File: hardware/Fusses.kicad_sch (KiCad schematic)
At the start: 8 parts, among them U16 FOD8802DR2, U17 FOD8802DR2

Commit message: changed some footprints for clarity, and made some progress on board
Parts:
- removed D10, D9: D_SCH, Diode_SMD:D_0603_1608Metric, symbol Device:D_Schottky_Small
- removed R17, R18, R41, R42: R_Small, Resistor_SMD:R_0603_1608Metric, symbol Device:R_Small
- removed U16, U17: FOD8802DR2, SOIC127P600X175-8N, symbol FOD8802DR2:FOD8802DR2
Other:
- added sheet Supply (eFuse supply 24V.kicad_sch)
- note added: "Smart Fuses 24V"
- note added: "eFuses 24V"
- note added: "eFuses 5V"
- note removed: "Fuses"

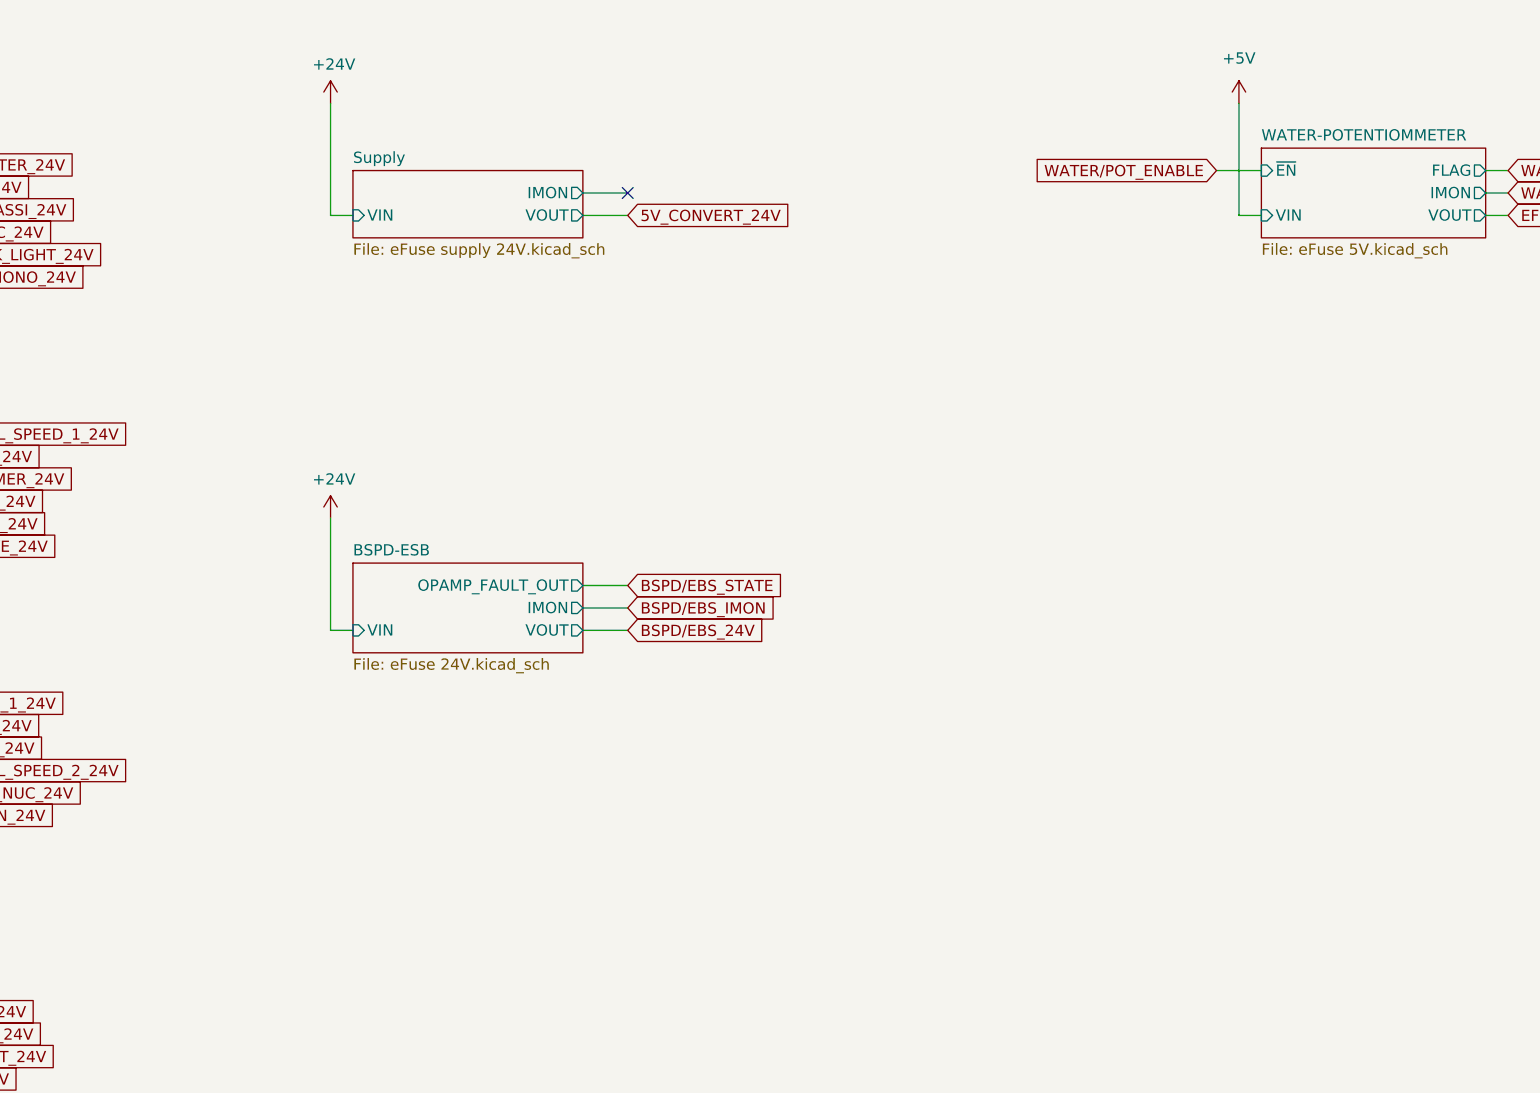
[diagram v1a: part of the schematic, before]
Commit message: finished new wersion of the board
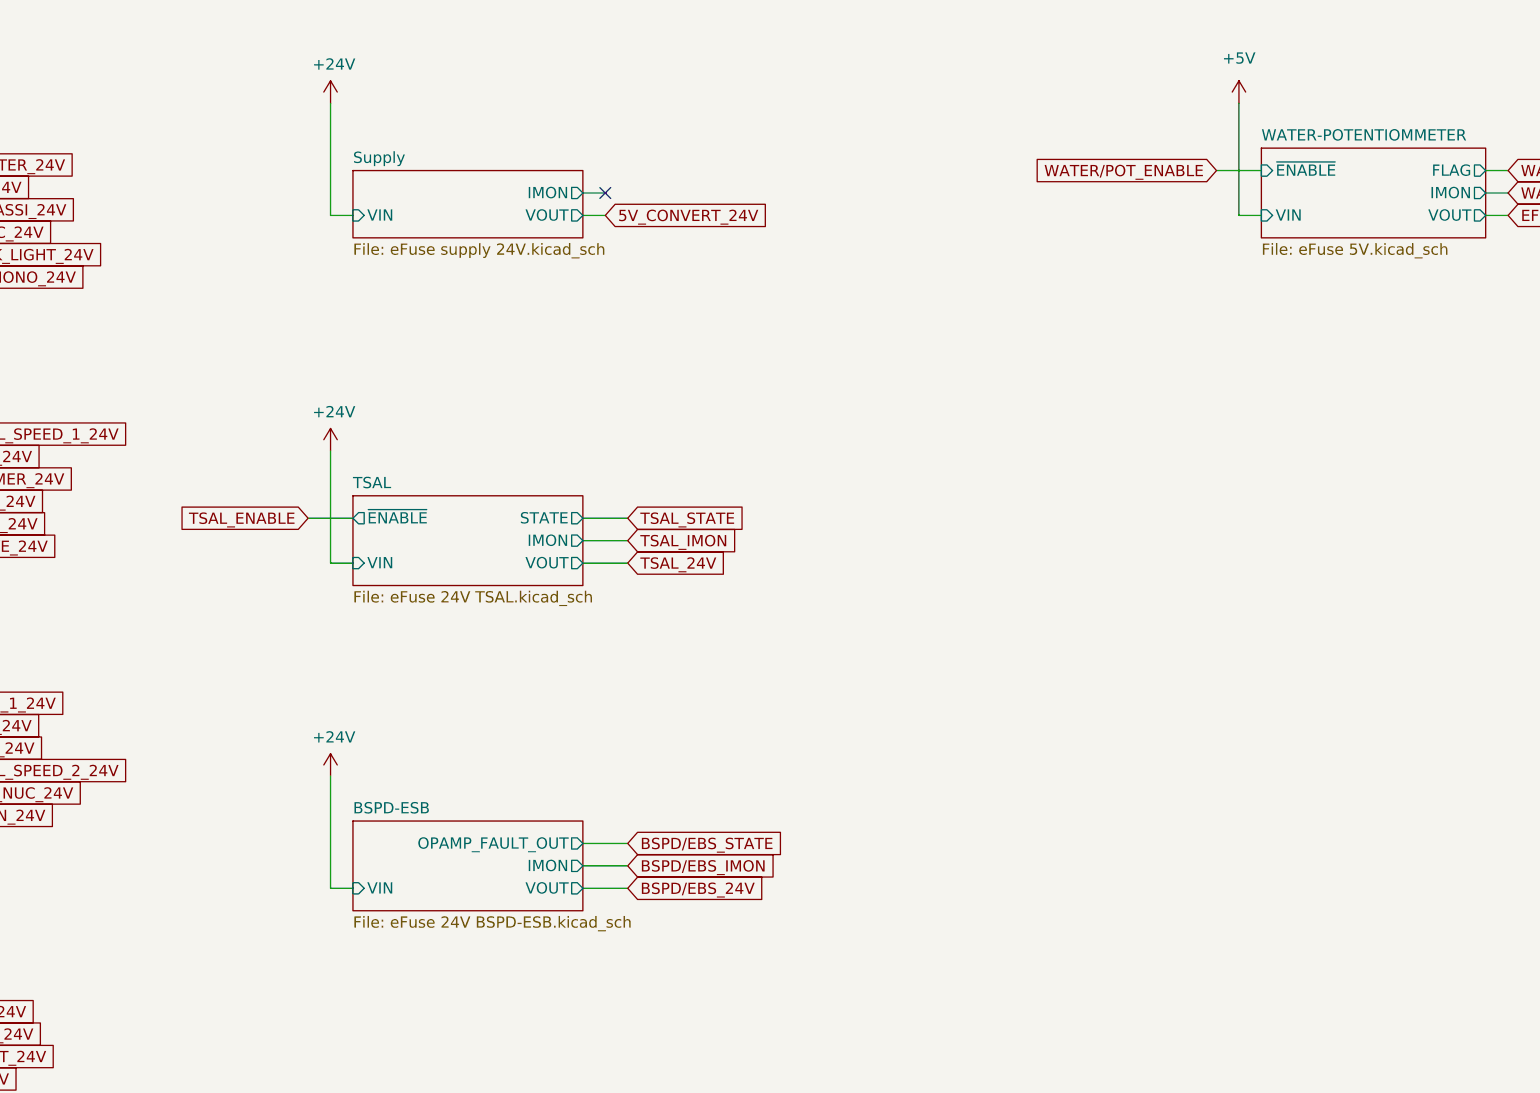
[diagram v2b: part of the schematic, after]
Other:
- added sheet TSAL (eFuse 24V TSAL.kicad_sch)
- sheet BSPD-ESB: file eFuse 24V.kicad_sch -> eFuse 24V BSPD-ESB.kicad_sch
- sheet WATER-POTENTIOMMETER ports: added ~{ENABLE}; removed ~{EN}
